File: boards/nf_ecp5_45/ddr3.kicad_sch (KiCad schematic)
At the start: 63 parts, among them U1 ECP5U_25_CABGA256, U11 AS4C256M16D3, U2 TPS51200DRC, U3 AS4C256M16D3

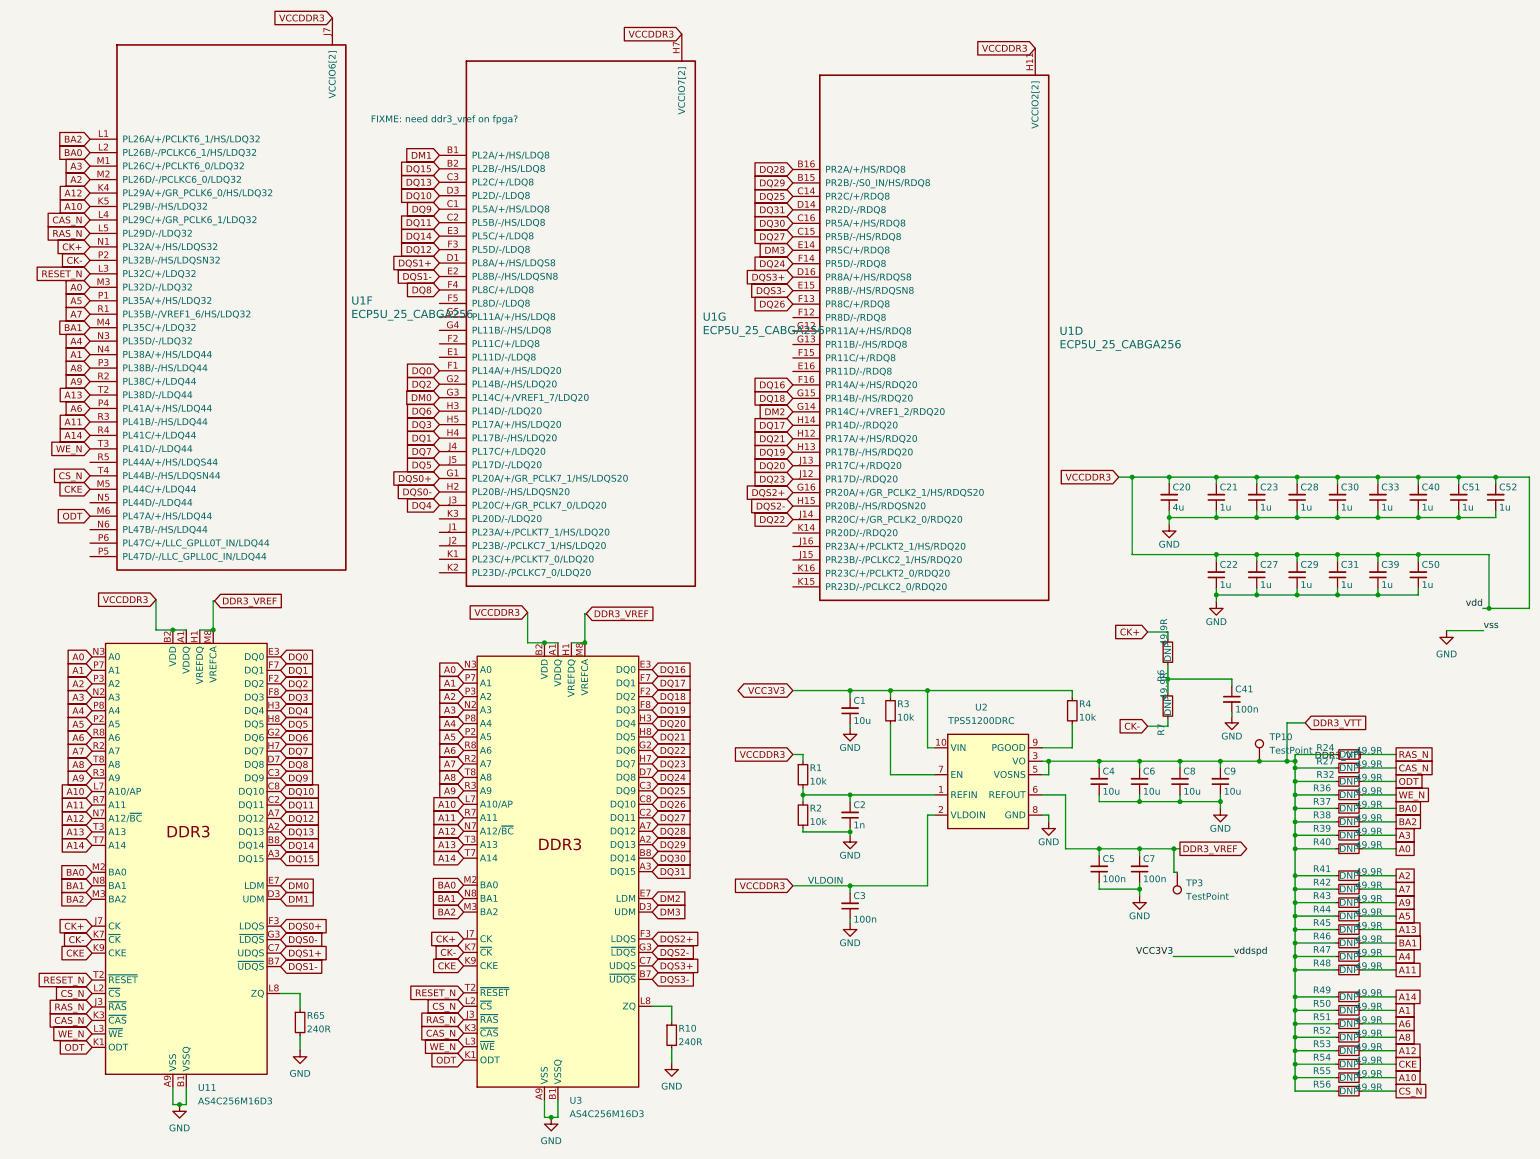
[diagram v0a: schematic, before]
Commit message: board
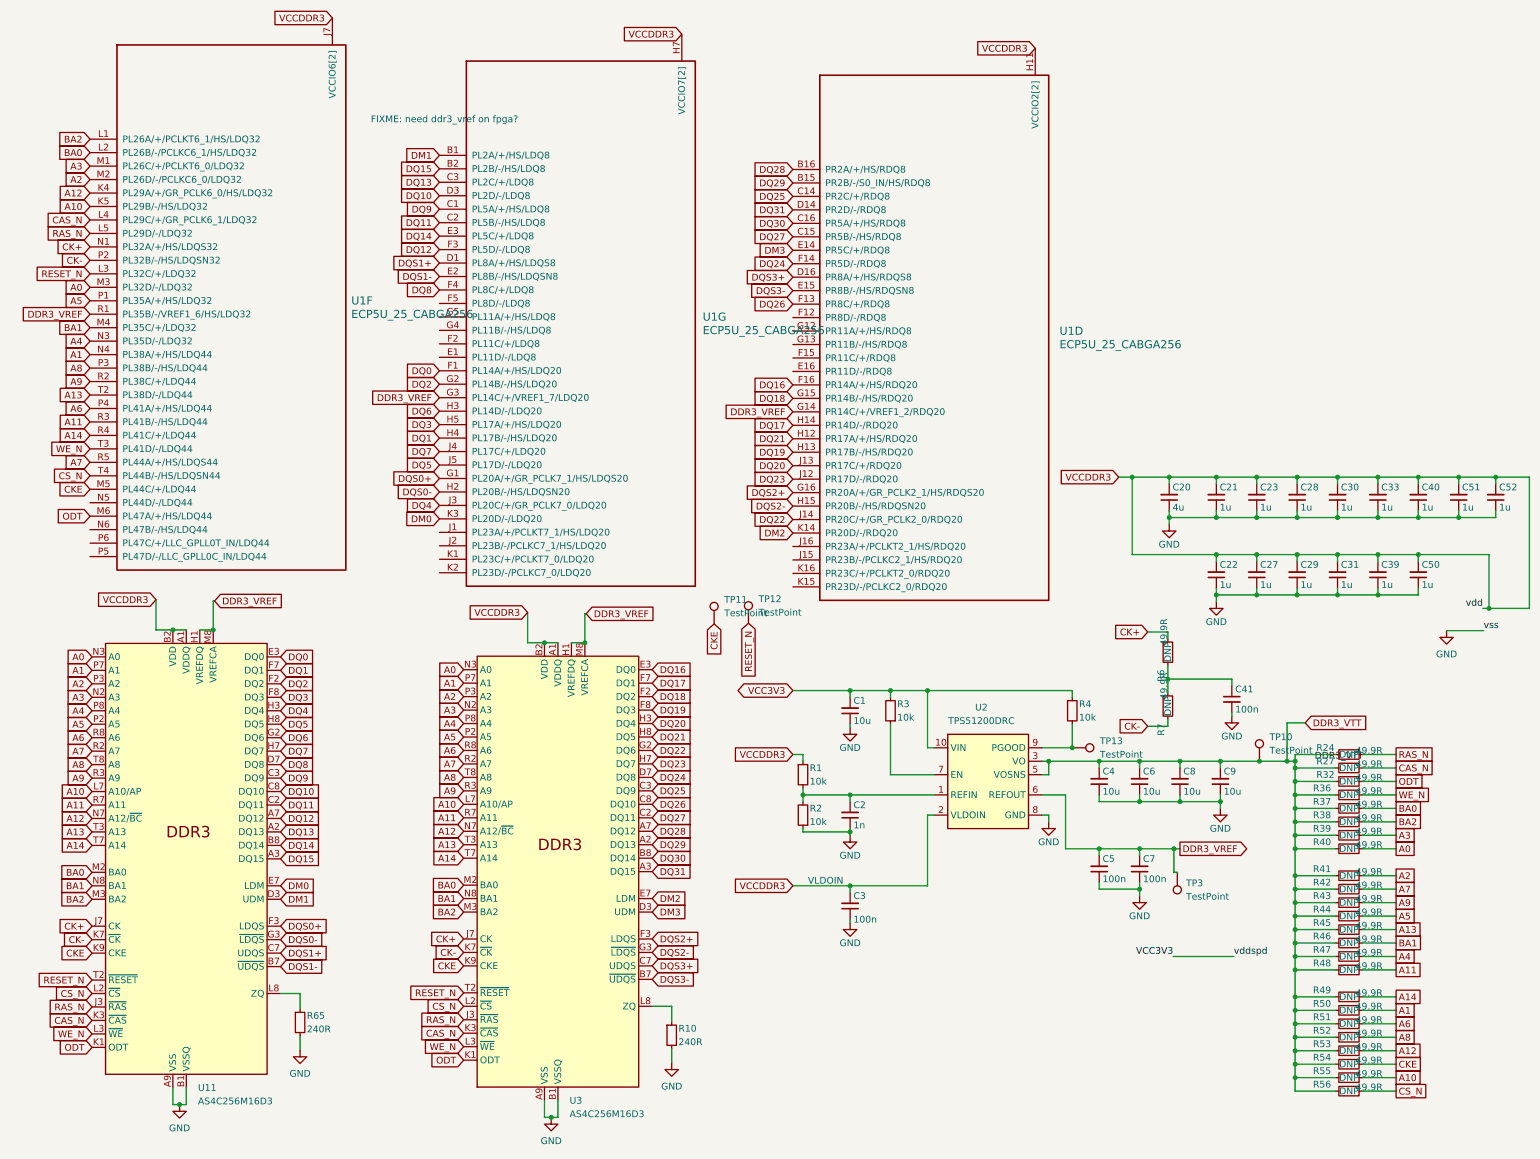
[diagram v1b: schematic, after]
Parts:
- added TP11, TP12, TP13: TestPoint, TestPoint:TestPoint_Pad_D1.0mm, symbol Connector:TestPoint
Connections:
- net A7: now also U1.R5 (PL44A/+/HS/LDQS44); no longer U1.R1 (PL35B/-/VREF1_6/HS/LDQ32)
- net CKE: now also TP11.1
- net DDR3_VREF: now also U1.G14 (PR14C/+/VREF1_2/RDQ20), U1.G3 (PL14C/+/VREF1_7/LDQ20), U1.R1 (PL35B/-/VREF1_6/HS/LDQ32)
- net DM0: now also U1.K3 (PL20D/-/LDQ20); no longer U1.G3 (PL14C/+/VREF1_7/LDQ20)
- net DM2: now also U1.K14 (PR20D/-/RDQ20); no longer U1.G14 (PR14C/+/VREF1_2/RDQ20)
- net RESET_N: now also TP12.1
- net at R4.2, U2.9 (PGOOD): now also TP13.1
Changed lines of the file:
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@@
   (junction (at 169.926 129.794) (diameter 0) (color 0 0 0 0)
   )
+  (junction (at 211.836 140.589) (diameter 0) (color 0 0 0 0)
+  )
   (junction (at 119.888 120.777) (diameter 0) (color 0 0 0 0)
   )
@@
     )
   )
+  (global_label "DDR3_VREF" (shape input) (at 92.456 74.549 180) (fields_autoplaced)
+    (effects (font (size 1.27 1.27)) (justify right))
+    (property "Intersheetrefs" "${INTERSHEET_REFS}" (at 78.8875 74.549 0)
+      (effects (font (size 1.27 1.27)) (justify right) hide)
+    )
+  )
   (global_label "A13" (shape input) (at 97.028 158.877 180) (fields_autoplaced)
     (effects (font (size 1.27 1.27)) (justify right))
@@
     )
   )
+  (global_label "CKE" (shape input) (at 144.272 117.221 270) (fields_autoplaced)
+    (effects (font (size 1.27 1.27)) (justify right))
+    (property "Intersheetrefs" "${INTERSHEET_REFS}" (at 144.272 123.8952 90)
+      (effects (font (size 1.27 1.27)) (justify right) hide)
+    )
+  )
   (global_label "DQ11" (shape input) (at 92.456 41.529 180) (fields_autoplaced)
     (effects (font (size 1.27 1.27)) (justify right))
@@
     )
   )
-  (global_label "A7" (shape input) (at 26.543 58.801 180) (fields_autoplaced)
+  (global_label "A7" (shape input) (at 26.543 86.741 180) (fields_autoplaced)
     (effects (font (size 1.27 1.27)) (justify right))
-    (property "Intersheetrefs" "${INTERSHEET_REFS}" (at 21.2597 58.801 0)
+    (property "Intersheetrefs" "${INTERSHEET_REFS}" (at 21.2597 86.741 0)
       (effects (font (size 1.27 1.27)) (justify right) hide)
     )
@@
     )
   )
-  (global_label "DM0" (shape input) (at 92.456 74.549 180) (fields_autoplaced)
+  (global_label "DM0" (shape input) (at 92.456 97.409 180) (fields_autoplaced)
     (effects (font (size 1.27 1.27)) (justify right))
-    (property "Intersheetrefs" "${INTERSHEET_REFS}" (at 85.5399 74.549 0)
+    (property "Intersheetrefs" "${INTERSHEET_REFS}" (at 85.5399 97.409 0)
       (effects (font (size 1.27 1.27)) (justify right) hide)
     )
@@
     )
   )
-  (global_label "DM2" (shape input) (at 159.131 77.216 180) (fields_autoplaced)
+  (global_label "DM2" (shape input) (at 159.131 100.076 180) (fields_autoplaced)
     (effects (font (size 1.27 1.27)) (justify right))
-    (property "Intersheetrefs" "${INTERSHEET_REFS}" (at 152.2149 77.216 0)
+    (property "Intersheetrefs" "${INTERSHEET_REFS}" (at 152.2149 100.076 0)
       (effects (font (size 1.27 1.27)) (justify right) hide)
     )
@@
     )
   )
+  (global_label "RESET_N" (shape input) (at 150.749 117.094 270) (fields_autoplaced)
+    (effects (font (size 1.27 1.27)) (justify right))
+    (property "Intersheetrefs" "${INTERSHEET_REFS}" (at 150.749 128.1224 90)
+      (effects (font (size 1.27 1.27)) (justify right) hide)
+    )
+  )
   (global_label "DQS3+" (shape input) (at 159.131 51.816 180) (fields_autoplaced)
     (effects (font (size 1.27 1.27)) (justify right))
@@
     )
   )
+  (global_label "DDR3_VREF" (shape input) (at 159.131 77.216 180) (fields_autoplaced)
+    (effects (font (size 1.27 1.27)) (justify right))
+    (property "Intersheetrefs" "${INTERSHEET_REFS}" (at 145.5625 77.216 0)
+      (effects (font (size 1.27 1.27)) (justify right) hide)
+    )
+  )
   (global_label "A11" (shape input) (at 97.028 153.797 180) (fields_autoplaced)
     (effects (font (size 1.27 1.27)) (justify right))
@@
     )
   )
+  (global_label "DDR3_VREF" (shape input) (at 26.543 58.801 180) (fields_autoplaced)
+    (effects (font (size 1.27 1.27)) (justify right))
+    (property "Intersheetrefs" "${INTERSHEET_REFS}" (at 12.9745 58.801 0)
+      (effects (font (size 1.27 1.27)) (justify right) hide)
+    )
+  )
   (global_label "A10" (shape input) (at 26.924 148.844 180) (fields_autoplaced)
     (effects (font (size 1.27 1.27)) (justify right))
@@
     )
   )
+  (symbol (lib_id "Connector:TestPoint") (at 211.836 140.589 270) (unit 1)
+    (in_bom yes) (on_board yes) (dnp no) (fields_autoplaced)
+    (property "Reference" "TP13" (at 217.043 139.319 90)
+      (effects (font (size 1.27 1.27)) (justify left))
+    )
+    (property "Value" "TestPoint" (at 217.043 141.859 90)
+      (effects (font (size 1.27 1.27)) (justify left))
+    )
+    (property "Footprint" "TestPoint:TestPoint_Pad_D1.0mm" (at 211.836 145.669 0)
+      (effects (font (size 1.27 1.27)) hide)
+    )
+    (property "Datasheet" "~" (at 211.836 145.669 0)
+      (effects (font (size 1.27 1.27)) hide)
+    )
+    (pin "1")
+    (instances
+      (project "nf_tpu"
+        (path "/9bed7131-c603-46c6-ae3c-0e9faa418ea0/b780d3b5-6a01-46cb-b503-97403d95c26a"
+          (reference "TP13") (unit 1)
+        )
+      )
+    )
+  )
   (symbol (lib_name "R_51R_0402_18") (lib_id "antmicroResistors0402:R_51R_0402") (at 266.573 144.399 0) (mirror y) (unit 1)
     (in_bom yes) (on_board yes) (dnp no)
@@
     )
   )
+  (symbol (lib_id "Connector:TestPoint") (at 150.749 117.094 0) (unit 1)
+    (in_bom yes) (on_board yes) (dnp no) (fields_autoplaced)
+    (property "Reference" "TP12" (at 152.654 112.522 0)
+      (effects (font (size 1.27 1.27)) (justify left))
+    )
+    (property "Value" "TestPoint" (at 152.654 115.062 0)
+      (effects (font (size 1.27 1.27)) (justify left))
+    )
+    (property "Footprint" "TestPoint:TestPoint_Pad_D1.0mm" (at 155.829 117.094 0)
+      (effects (font (size 1.27 1.27)) hide)
+    )
+    (property "Datasheet" "~" (at 155.829 117.094 0)
+      (effects (font (size 1.27 1.27)) hide)
+    )
+    (pin "1")
+    (instances
+      (project "nf_tpu"
+        (path "/9bed7131-c603-46c6-ae3c-0e9faa418ea0/b780d3b5-6a01-46cb-b503-97403d95c26a"
+          (reference "TP12") (unit 1)
+        )
+      )
+    )
+  )
   (symbol (lib_name "R_51R_0402_6") (lib_id "antmicroResistors0402:R_51R_0402") (at 266.573 167.259 0) (mirror y) (unit 1)
     (in_bom yes) (on_board yes) (dnp no)
@@
         )
       )
+    )
+  )
+  (symbol (lib_id "Connector:TestPoint") (at 144.272 117.221 0) (unit 1)
+    (in_bom yes) (on_board yes) (dnp no) (fields_autoplaced)
+    (property "Reference" "TP11" (at 146.177 112.649 0)
+      (effects (font (size 1.27 1.27)) (justify left))
+    )
+    (property "Value" "TestPoint" (at 146.177 115.189 0)
+      (effects (font (size 1.27 1.27)) (justify left))
+    )
+    (property "Footprint" "TestPoint:TestPoint_Pad_D1.0mm" (at 149.352 117.221 0)
+      (effects (font (size 1.27 1.27)) hide)
+    )
+    (property "Datasheet" "~" (at 149.352 117.221 0)
+      (effects (font (size 1.27 1.27)) hide)
+    )
+    (pin "1")
+    (instances
+      (project "nf_tpu"
+        (path "/9bed7131-c603-46c6-ae3c-0e9faa418ea0/b780d3b5-6a01-46cb-b503-97403d95c26a"
+          (reference "TP11") (unit 1)
+        )
+      )

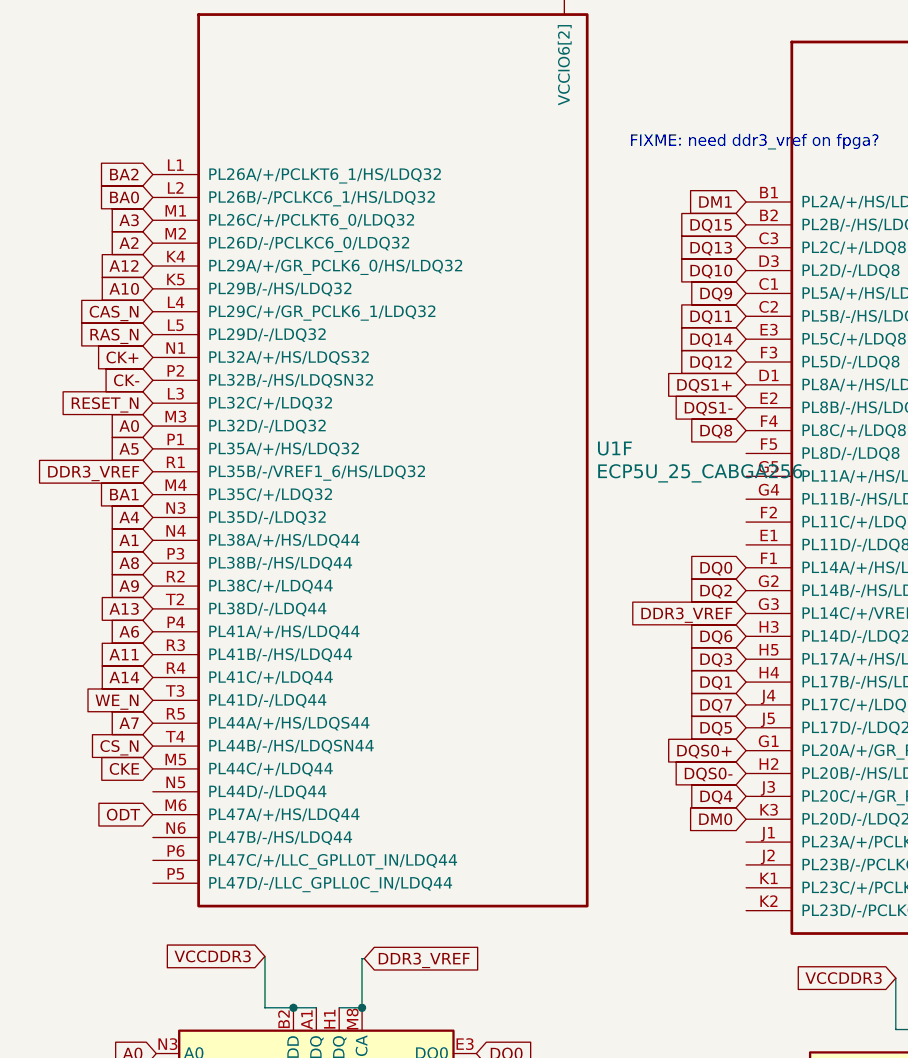
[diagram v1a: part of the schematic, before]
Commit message: board
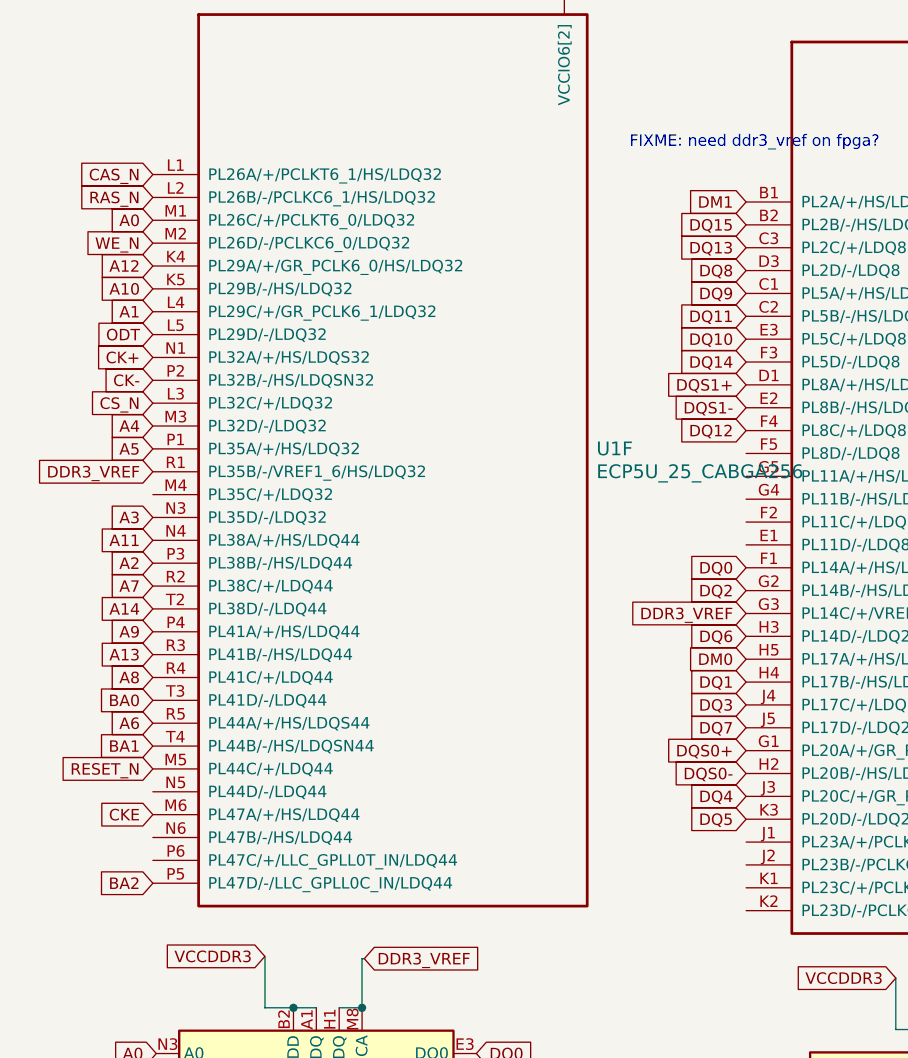
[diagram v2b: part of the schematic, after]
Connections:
- net A0: now also U1.M1 (PL26C/+/PCLKT6_0/LDQ32); no longer U1.M3 (PL32D/-/LDQ32)
- net A1: now also U1.L4 (PL29C/+/GR_PCLK6_1/LDQ32); no longer U1.N4 (PL38A/+/HS/LDQ44)
- net A11: now also U1.N4 (PL38A/+/HS/LDQ44); no longer U1.R3 (PL41B/-/HS/LDQ44)
- net A13: now also U1.R3 (PL41B/-/HS/LDQ44); no longer U1.T2 (PL38D/-/LDQ44)
- net A14: now also U1.T2 (PL38D/-/LDQ44); no longer U1.R4 (PL41C/+/LDQ44)
- net A2: now also U1.P3 (PL38B/-/HS/LDQ44); no longer U1.M2 (PL26D/-/PCLKC6_0/LDQ32)
- net A3: now also U1.N3 (PL35D/-/LDQ32); no longer U1.M1 (PL26C/+/PCLKT6_0/LDQ32)
- net A4: now also U1.M3 (PL32D/-/LDQ32); no longer U1.N3 (PL35D/-/LDQ32)
- net A6: now also U1.R5 (PL44A/+/HS/LDQS44); no longer U1.P4 (PL41A/+/HS/LDQ44)
- net A7: now also U1.R2 (PL38C/+/LDQ44); no longer U1.R5 (PL44A/+/HS/LDQS44)
- net A8: now also U1.R4 (PL41C/+/LDQ44); no longer U1.P3 (PL38B/-/HS/LDQ44)
- net A9: now also U1.P4 (PL41A/+/HS/LDQ44); no longer U1.R2 (PL38C/+/LDQ44)
- net BA0: now also U1.T3 (PL41D/-/LDQ44); no longer U1.L2 (PL26B/-/PCLKC6_1/HS/LDQ32)
- net BA1: now also U1.T4 (PL44B/-/HS/LDQSN44); no longer U1.M4 (PL35C/+/LDQ32)
- net BA2: now also U1.P5 (PL47D/-/LLC_GPLL0C_IN/LDQ44); no longer U1.L1 (PL26A/+/PCLKT6_1/HS/LDQ32)
- net CAS_N: now also U1.L1 (PL26A/+/PCLKT6_1/HS/LDQ32); no longer U1.L4 (PL29C/+/GR_PCLK6_1/LDQ32)
- net CKE: now also U1.M6 (PL47A/+/HS/LDQ44); no longer U1.M5 (PL44C/+/LDQ44)
- net CS_N: now also U1.L3 (PL32C/+/LDQ32); no longer U1.T4 (PL44B/-/HS/LDQSN44)
- net DM0: now also U1.H5 (PL17A/+/HS/LDQ20); no longer U1.K3 (PL20D/-/LDQ20)
- net DQ10: now also U1.E3 (PL5C/+/LDQ8); no longer U1.D3 (PL2D/-/LDQ8)
- net DQ12: now also U1.F4 (PL8C/+/LDQ8); no longer U1.F3 (PL5D/-/LDQ8)
- net DQ14: now also U1.F3 (PL5D/-/LDQ8); no longer U1.E3 (PL5C/+/LDQ8)
- net DQ3: now also U1.J4 (PL17C/+/LDQ20); no longer U1.H5 (PL17A/+/HS/LDQ20)
- net DQ5: now also U1.K3 (PL20D/-/LDQ20); no longer U1.J5 (PL17D/-/LDQ20)
- net DQ7: now also U1.J5 (PL17D/-/LDQ20); no longer U1.J4 (PL17C/+/LDQ20)
- net DQ8: now also U1.D3 (PL2D/-/LDQ8); no longer U1.F4 (PL8C/+/LDQ8)
- net ODT: now also U1.L5 (PL29D/-/LDQ32); no longer U1.M6 (PL47A/+/HS/LDQ44)
- net RAS_N: now also U1.L2 (PL26B/-/PCLKC6_1/HS/LDQ32); no longer U1.L5 (PL29D/-/LDQ32)
- net RESET_N: now also U1.M5 (PL44C/+/LDQ44); no longer U1.L3 (PL32C/+/LDQ32)
- net WE_N: now also U1.M2 (PL26D/-/PCLKC6_0/LDQ32); no longer U1.T3 (PL41D/-/LDQ44)
